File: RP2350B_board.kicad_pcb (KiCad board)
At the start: 2 copper layers, 47.5 x 66 mm, 45 parts, among them IC1 W25Q128JVSIM, IC2 UA78M33CDCYG3, J1 USB_C_Receptacle_USB2.0_16P, J2 SWD, J3 Conn_01x25_Pin, J4 Conn_01x25_Pin, J5 Conn_01x25_Pin, J6 Conn_01x25_Pin, J7 Conn_01x25_Pin, J8 Conn_01x25_Pin, U1 RP2350_80QFN, Y1 ABM8-272-T3

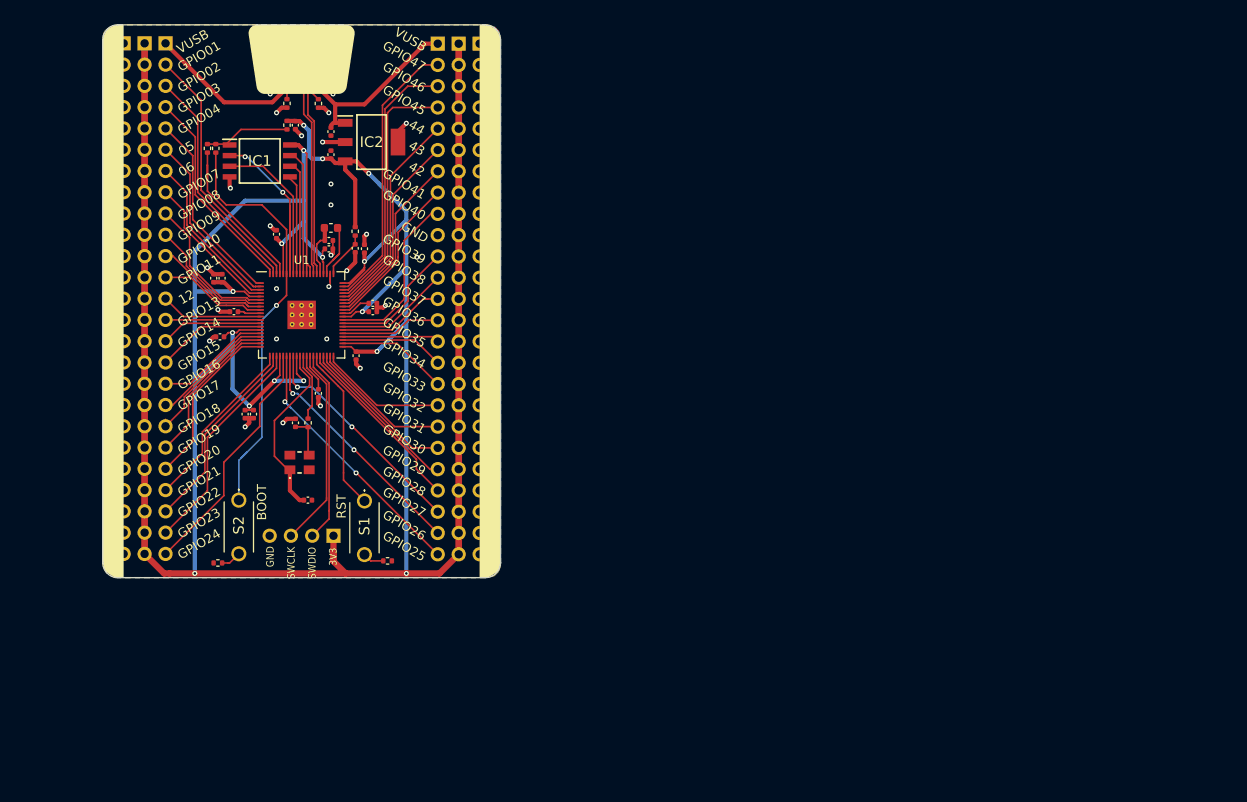
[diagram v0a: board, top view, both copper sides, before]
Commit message: refactor: start new layout
Signed-off-by: Aditya Agarwal <aditya.agarwal030504@gmail.com>
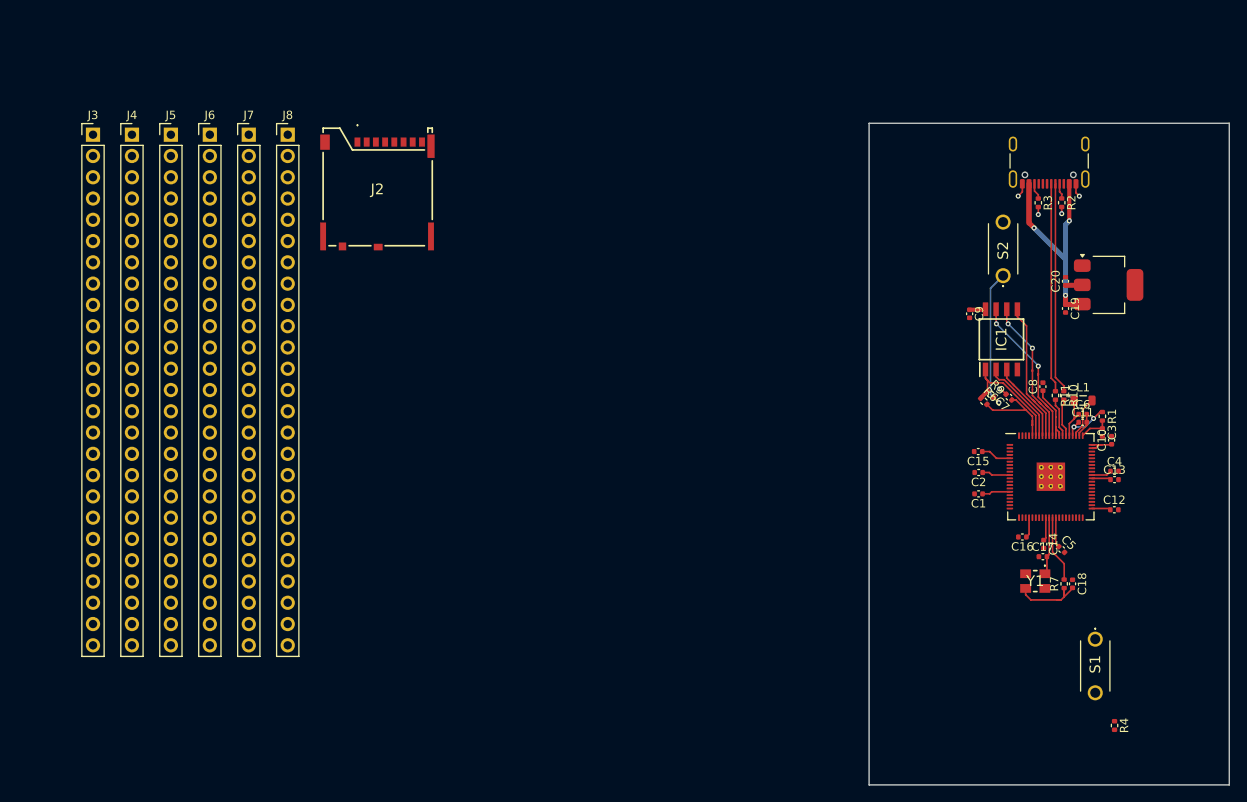
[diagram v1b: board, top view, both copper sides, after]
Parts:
- removed G***: LOGO, Dumblebots-Logo:Dumblebots-Logo
- removed IC2: UA78M33CDCYG3, UA78M33CDCYG3:SOT230P700X180-4N
- removed R5: 0, Resistor_SMD:R_0402_1005Metric
- removed R8: 1K, Resistor_SMD:R_0402_1005Metric
- added R10: 27, Resistor_SMD:R_0402_1005Metric, F.Cu at (237.2, 104.0)
- added R11: 27, Resistor_SMD:R_0402_1005Metric, F.Cu at (236.2, 104.0)
- added U2: NCP1117-3.3_SOT223, Package_TO_SOT_SMD:SOT-223-3_TabPin2, F.Cu at (242.6, 90.8)
- C19, C20: value 100n -> 10u
- J2: value SWD -> MEM2080-00-128-00-A; footprint Connector_PinHeader_2.54mm:PinHeader_1x04_P2.54mm_Vertical -> MEM2080-00-128-00-A:MEM20800012800A
- L1: footprint Inductor_SMD:L_0603_1608Metric -> Inductor_SMD:L_0805_2012Metric
- R4: value 10K -> 1K
- R6: value DNF -> 10K
- moved R4 122.1 mm to (243.3, 143.4), turned to -90 degrees
- moved C13 108.2 mm to (243.3, 114.0), turned to 0 degrees
- moved C12 104.4 mm to (243.3, 117.7), turned to 0 degrees
- moved C14 104.1 mm to (234.8, 121.8), turned to -90 degrees
- moved C6 102.1 mm to (239.5, 106.2), turned to 0 degrees
- moved C16 99.8 mm to (232.3, 120.9), turned to 180 degrees
- moved C11 99.0 mm to (239.5, 107.2), turned to 0 degrees
- moved R6 97.5 mm to (227.7, 104.7), turned to -45 degrees
- moved C3 95.2 mm to (241.8, 108.4), turned to -90 degrees
- moved S2 95.1 mm to (230.0, 89.7), turned to 90 degrees
- moved C18 94.7 mm to (238.3, 126.5), turned to -90 degrees
- moved R9 94.4 mm to (228.5, 103.9), turned to -45 degrees
- moved C15 92.6 mm to (227.0, 110.7), turned to 180 degrees
- moved R7 92.3 mm to (237.3, 126.5)
- moved L1 92.1 mm to (239.6, 104.6)
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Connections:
- net /VREG_LX renamed VREG_LX
- net Net-(U1-XOUT) renamed XOUT
- C1 pad 1: /VREG_AVDD -> IOVDD
- C1 pad 2: GND -> VREG_PGND
- C10 pad 1: +3.3v -> IOVDD
- C10 pad 2: GND -> VREG_PGND
- C11 pad 1: +3.3v -> IOVDD
- C11 pad 2: GND -> VREG_PGND
- C12 pad 1: +3.3v -> IOVDD
- C12 pad 2: GND -> VREG_PGND
- C13 pad 1: +3.3v -> IOVDD
- C13 pad 2: GND -> VREG_PGND
- C14 pad 1: +3.3v -> IOVDD
- C14 pad 2: GND -> VREG_PGND
- C15 pad 1: +3.3v -> IOVDD
- C15 pad 2: GND -> VREG_PGND
- C16 pad 1: +3.3v -> IOVDD
- C16 pad 2: GND -> VREG_PGND
- C17 pad 1: Net-(U1-XIN) -> VREG_PGND
- C17 pad 2: GND -> XIN
- C18 pad 1: Net-(Y1-CRYSTAL_2) -> VREG_PGND
- C18 pad 2: GND -> Net-(C18-Pad2)
- C19 pad 2: GND -> VREG_PGND
- C2 pad 1: +3.3v -> DVDD
- C2 pad 2: GND -> VREG_PGND
- C20 pad 1: GND -> IOVDD
- C20 pad 2: +3.3v -> VREG_PGND
- C3 pad 1: +1V1 -> VREG_AVDD
- C3 pad 2: GND -> VREG_PGND
- C4 pad 1: +1V1 -> DVDD
- C4 pad 2: GND -> VREG_PGND
- C5 pad 1: +1V1 -> DVDD
- C5 pad 2: GND -> VREG_PGND
- C6 pad 1: +1V1 -> DVDD
- C6 pad 2: GND -> VREG_PGND
- C7 pad 1: +3.3v -> IOVDD
- C7 pad 2: GND -> VREG_PGND
- C8 pad 1: +3.3v -> IOVDD
- C8 pad 2: GND -> VREG_PGND
- C9 pad 1: +3.3v -> IOVDD
- C9 pad 2: GND -> VREG_PGND
- IC1 pad 1: Net-(IC1-~{CS}) -> GPIO0
- IC1 pad 4: GND -> VREG_PGND
- IC1 pad 8: +3.3v -> IOVDD
- J1 pad A1: GND -> VREG_PGND
- J1 pad A12: GND -> VREG_PGND
- J1 pad A6: USB_D+ -> Net-(J1-D+-PadA6)
- J1 pad A7: USB_D- -> Net-(J1-D--PadA7)
- J1 pad B1: GND -> VREG_PGND
- J1 pad B12: GND -> VREG_PGND
- J1 pad B6: USB_D+ -> Net-(J1-D+-PadA6)
- J1 pad B7: USB_D- -> Net-(J1-D--PadA7)
- J1 pad S1: GND -> VREG_PGND
- J2 pad 1: +3.3v -> unconnected-(J2-DAT2-Pad1)
- J2 pad 2: SWD -> unconnected-(J2-CD/DAT3-Pad2)
- J2 pad 3: SWCLK -> unconnected-(J2-CMD-Pad3)
- J2 pad 4: GND -> unconnected-(J2-VDD-Pad4)
- J4 pad 10: GND -> VREG_PGND
- J5 pad 1: GND -> VREG_PGND
- J5 pad 10: GND -> VREG_PGND
- J5 pad 11: GND -> VREG_PGND
- J5 pad 12: GND -> VREG_PGND
- J5 pad 13: GND -> VREG_PGND
- J5 pad 14: GND -> VREG_PGND
- J5 pad 15: GND -> VREG_PGND
- J5 pad 16: GND -> VREG_PGND
- J5 pad 17: GND -> VREG_PGND
- J5 pad 18: GND -> VREG_PGND
- J5 pad 19: GND -> VREG_PGND
- J5 pad 2: GND -> VREG_PGND
- J5 pad 20: GND -> VREG_PGND
- J5 pad 21: GND -> VREG_PGND
- J5 pad 22: GND -> VREG_PGND
- J5 pad 23: GND -> VREG_PGND
- J5 pad 24: GND -> VREG_PGND
- J5 pad 25: GND -> VREG_PGND
- J5 pad 3: GND -> VREG_PGND
- J5 pad 4: GND -> VREG_PGND
- J5 pad 5: GND -> VREG_PGND
- J5 pad 6: GND -> VREG_PGND
- J5 pad 7: GND -> VREG_PGND
- J5 pad 8: GND -> VREG_PGND
- J5 pad 9: GND -> VREG_PGND
- J6 pad 1: GND -> VREG_PGND
- J6 pad 10: GND -> VREG_PGND
- J6 pad 11: GND -> VREG_PGND
- J6 pad 12: GND -> VREG_PGND
- J6 pad 13: GND -> VREG_PGND
- J6 pad 14: GND -> VREG_PGND
- J6 pad 15: GND -> VREG_PGND
- J6 pad 16: GND -> VREG_PGND
- J6 pad 17: GND -> VREG_PGND
- J6 pad 18: GND -> VREG_PGND
- J6 pad 19: GND -> VREG_PGND
- J6 pad 2: GND -> VREG_PGND
- J6 pad 20: GND -> VREG_PGND
- J6 pad 21: GND -> VREG_PGND
- J6 pad 22: GND -> VREG_PGND
- J6 pad 23: GND -> VREG_PGND
- J6 pad 24: GND -> VREG_PGND
- J6 pad 25: GND -> VREG_PGND
- J6 pad 3: GND -> VREG_PGND
- J6 pad 4: GND -> VREG_PGND
- J6 pad 5: GND -> VREG_PGND
- J6 pad 6: GND -> VREG_PGND
- J6 pad 7: GND -> VREG_PGND
- J6 pad 8: GND -> VREG_PGND
- J6 pad 9: GND -> VREG_PGND
- J7 pad 1: +3.3v -> IOVDD
- J7 pad 10: +3.3v -> IOVDD
- J7 pad 11: +3.3v -> IOVDD
- J7 pad 12: +3.3v -> IOVDD
- J7 pad 13: +3.3v -> IOVDD
- J7 pad 14: +3.3v -> IOVDD
- J7 pad 15: +3.3v -> IOVDD
- J7 pad 16: +3.3v -> IOVDD
- J7 pad 17: +3.3v -> IOVDD
- J7 pad 18: +3.3v -> IOVDD
- J7 pad 19: +3.3v -> IOVDD
- J7 pad 2: +3.3v -> IOVDD
- J7 pad 20: +3.3v -> IOVDD
- J7 pad 21: +3.3v -> IOVDD
- J7 pad 22: +3.3v -> IOVDD
- J7 pad 23: +3.3v -> IOVDD
- J7 pad 24: +3.3v -> IOVDD
- J7 pad 25: +3.3v -> IOVDD
- J7 pad 3: +3.3v -> IOVDD
- J7 pad 4: +3.3v -> IOVDD
- J7 pad 5: +3.3v -> IOVDD
- J7 pad 6: +3.3v -> IOVDD
- J7 pad 7: +3.3v -> IOVDD
- J7 pad 8: +3.3v -> IOVDD
- J7 pad 9: +3.3v -> IOVDD
- J8 pad 1: +3.3v -> IOVDD
- J8 pad 10: +3.3v -> IOVDD
- J8 pad 11: +3.3v -> IOVDD
- J8 pad 12: +3.3v -> IOVDD
- J8 pad 13: +3.3v -> IOVDD
- J8 pad 14: +3.3v -> IOVDD
- J8 pad 15: +3.3v -> IOVDD
- J8 pad 16: +3.3v -> IOVDD
- J8 pad 17: +3.3v -> IOVDD
- J8 pad 18: +3.3v -> IOVDD
- J8 pad 19: +3.3v -> IOVDD
- J8 pad 2: +3.3v -> IOVDD
- J8 pad 20: +3.3v -> IOVDD
- J8 pad 21: +3.3v -> IOVDD
- J8 pad 22: +3.3v -> IOVDD
- J8 pad 23: +3.3v -> IOVDD
- J8 pad 24: +3.3v -> IOVDD
- J8 pad 25: +3.3v -> IOVDD
- J8 pad 3: +3.3v -> IOVDD
- J8 pad 4: +3.3v -> IOVDD
- J8 pad 5: +3.3v -> IOVDD
- J8 pad 6: +3.3v -> IOVDD
- J8 pad 7: +3.3v -> IOVDD
- J8 pad 8: +3.3v -> IOVDD
- J8 pad 9: +3.3v -> IOVDD
- L1 pad 1: +1V1 -> DVDD
- R1 pad 1: +3.3v -> IOVDD
- R1 pad 2: /VREG_AVDD -> VREG_AVDD
- R2 pad 2: GND -> VREG_PGND
- R3 pad 2: GND -> VREG_PGND
- R4 pad 1: Net-(IC1-~{CS}) -> VREG_PGND
- R4 pad 2: +3.3v -> Net-(S1-NO)
- R6 pad 2: Net-(IC1-~{CS}) -> IOVDD
- R7 pad 1: Net-(Y1-CRYSTAL_2) -> Net-(C18-Pad2)
- R9 pad 1: GND -> GPIO0
- R9 pad 2: Net-(S2-NO) -> Net-(S2-COM)
- S2 pad 1: QSPI_SS -> Net-(S2-COM)
- S2 pad 2: Net-(S2-NO) -> VREG_PGND
- U1 pad 10: +1V1 -> DVDD
- U1 pad 15: +3.3v -> IOVDD
- U1 pad 24: +3.3v -> IOVDD
- U1 pad 29: +3.3v -> IOVDD
- U1 pad 30: Net-(U1-XIN) -> XIN
- U1 pad 32: +1V1 -> DVDD
- U1 pad 41: +3.3v -> IOVDD
- U1 pad 5: +3.3v -> IOVDD
- U1 pad 50: +3.3v -> IOVDD
- U1 pad 51: +1V1 -> DVDD
- U1 pad 59: +3.3v -> IOVDD
- U1 pad 60: +3.3v -> IOVDD
- U1 pad 61: /VREG_AVDD -> VREG_AVDD
- U1 pad 62: GND -> VREG_PGND
- U1 pad 64: +3.3v -> IOVDD
- U1 pad 65: +1V1 -> DVDD
- U1 pad 68: +3.3v -> IOVDD
- U1 pad 69: +3.3v -> IOVDD
- U1 pad 75: QSPI_SS -> GPIO0
- U1 pad 76: +3.3v -> IOVDD
- U1 pad 81: GND -> VREG_PGND
- Y1 pad 1: Net-(U1-XIN) -> XIN
- Y1 pad 2: GND -> VREG_PGND
- Y1 pad 3: Net-(Y1-CRYSTAL_2) -> Net-(C18-Pad2)
- Y1 pad 4: GND -> VREG_PGND
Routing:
- net +3.3v: track 421.7 -> 0.00 mm, vias 16 -> 0
- net QSPI_SS: track 50.9 -> 0.00 mm, vias 1 -> 0
- net IOVDD: track 0.00 -> 48.8 mm, vias 0 -> 2
- net GND: track 37.4 -> 0.00 mm, vias 27 -> 0
- net GPIO47: track 33.0 -> 0.00 mm
- net GPIO25: track 32.1 -> 0.00 mm, vias 2 -> 0
- net GPIO46: track 31.9 -> 0.00 mm
- net GPIO45: track 30.8 -> 0.00 mm
- net GPIO1: track 30.5 -> 0.00 mm
- net GPIO26: track 30.3 -> 0.00 mm, vias 2 -> 0
- net GPIO24: track 29.5 -> 0.00 mm
- net GPIO2: track 27.8 -> 0.00 mm
- net GPIO27: track 26.8 -> 0.00 mm, vias 2 -> 0
- net GPIO23: track 26.6 -> 0.00 mm
- net GPIO44: track 25.6 -> 0.00 mm
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- removed copper zone on B.Cu, net GND
- removed copper zone on F.Cu, net GND
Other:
- board size 47.5 x 66 mm -> 43 x 79 mm
- board text removed: "05"
- board text removed: "06"
- board text removed: "12"
- board text removed: "3V3"
- board text removed: "42"
- board text removed: "43"
- board text removed: "44"
- board text removed: "BOOT"
- board text removed: "Designed and manufactured in Bharat"
- board text removed: "GND"
- board text removed: "GPIO01"
- board text removed: "GPIO02"
- board text removed: "GPIO03"
- board text removed: "GPIO04"
- board text removed: "GPIO07"
- board text removed: "GPIO08"
- board text removed: "GPIO09"
- board text removed: "GPIO10"
- board text removed: "GPIO11"
- board text removed: "GPIO13"
- board text removed: "GPIO14"
- board text removed: "GPIO15"
- board text removed: "GPIO16"
- board text removed: "GPIO17"
- board text removed: "GPIO18"
- board text removed: "GPIO19"
- board text removed: "GPIO20"
- board text removed: "GPIO21"
- board text removed: "GPIO22"
- board text removed: "GPIO23"
- board text removed: "GPIO24"
- board text removed: "GPIO25"
- board text removed: "GPIO26"
- board text removed: "GPIO27"
- board text removed: "GPIO28"
- board text removed: "GPIO29"
- board text removed: "GPIO30"
- board text removed: "GPIO31"
- board text removed: "GPIO32"
- board text removed: "GPIO33"
- board text removed: "GPIO34"
- board text removed: "GPIO35"
- board text removed: "GPIO36"
- board text removed: "GPIO37"
- board text removed: "GPIO38"
- board text removed: "GPIO39"
- board text removed: "GPIO40"
- board text removed: "GPIO41"
- board text removed: "GPIO45"
- board text removed: "GPIO46"
- board text removed: "GPIO47"
- board text removed: "RP2350B Dev Board"
- board text removed: "RST"
- board text removed: "SWCLK"
- board text removed: "SWDIO"
- board text removed: "VUSB"
- board text removed: "dumblebots.com"

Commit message: feat: complete all features except SD Card reader
Signed-off-by: Aditya Agarwal <aditya.agarwal030504@gmail.com>
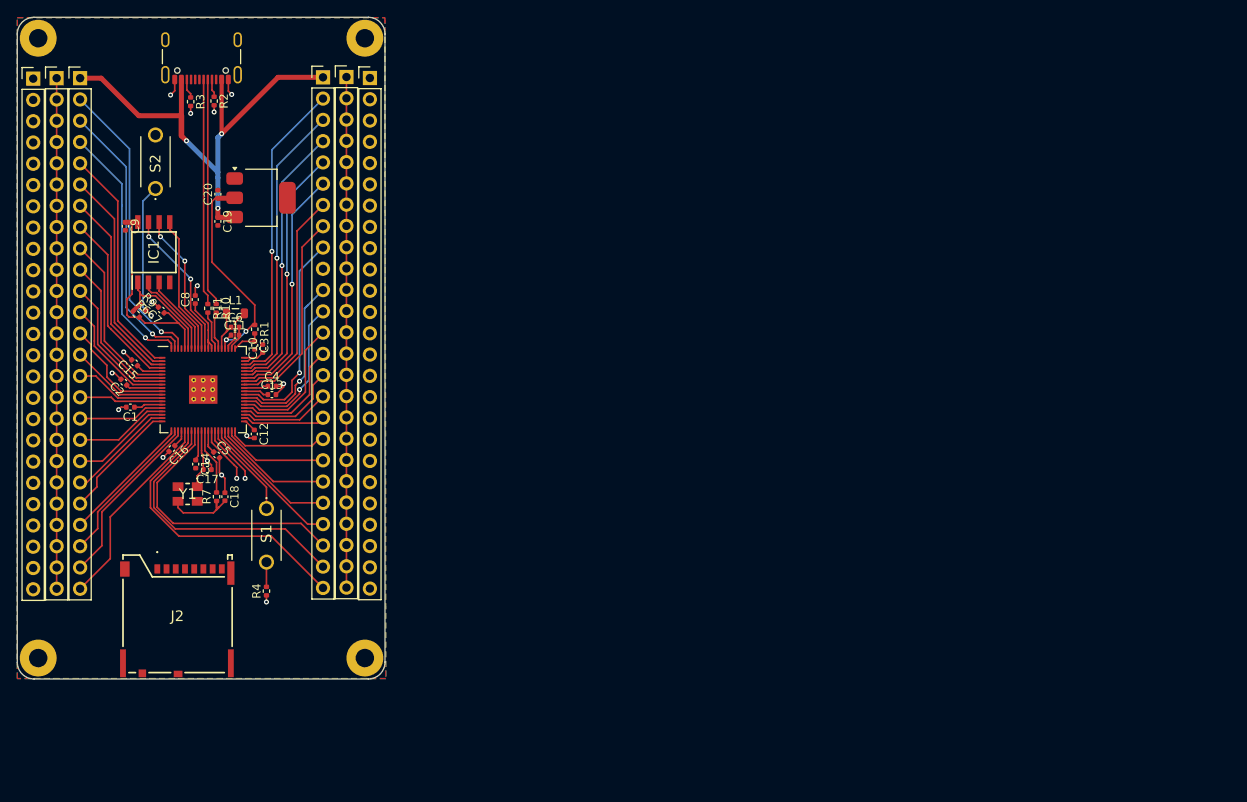
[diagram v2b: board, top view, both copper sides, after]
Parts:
- added REF**: MountingHole_2.2mm_M2_Pad, MountingHole:MountingHole_2.2mm_M2_Pad, F.Cu at (153.8, 135.3)
- added REF**: MountingHole_2.2mm_M2_Pad, MountingHole:MountingHole_2.2mm_M2_Pad, F.Cu at (114.8, 135.3)
- added REF**: MountingHole_2.2mm_M2_Pad, MountingHole:MountingHole_2.2mm_M2_Pad, F.Cu at (153.8, 61.4)
- added REF**: MountingHole_2.2mm_M2_Pad, MountingHole:MountingHole_2.2mm_M2_Pad, F.Cu at (114.8, 61.4)
- moved C12 103.1 mm to (140.6, 108.6), turned to -90 degrees
- moved C2 102.6 mm to (125.0, 102.4), turned to 135 degrees
- moved R4 102.5 mm to (142.1, 127.4), turned to 90 degrees
- moved C16 102.1 mm to (130.8, 110.3), turned to -135 degrees
- moved J1 102.0 mm to (134.3, 62.6)
- moved C10 101.9 mm to (141.6, 98.4)
- moved R2 101.9 mm to (135.8, 68.8)
- moved R3 101.9 mm to (133.0, 68.9)
- moved C1 101.8 mm to (125.8, 105.4)
- moved IC1 101.7 mm to (128.6, 86.9)
- moved L1 101.7 mm to (138.3, 94.2)
- moved Y1 101.7 mm to (132.6, 115.8)
- moved R9 101.7 mm to (127.3, 93.5)
- moved C11 101.7 mm to (138.3, 96.8)
- moved C18 101.7 mm to (137.1, 116.1)
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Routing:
- net IOVDD: track 48.8 -> 200.8 mm
- net GPIO47: track 0.00 -> 36.9 mm, vias 0 -> 1
- net GPIO25: track 0.00 -> 35.6 mm
- net GPIO1: track 0.00 -> 35.3 mm, vias 0 -> 1
- net GPIO46: track 0.00 -> 34.8 mm, vias 0 -> 1
- net GPIO26: track 0.00 -> 34.2 mm
- net GPIO2: track 0.00 -> 33.0 mm, vias 0 -> 1
- net VBUS: track 28.1 -> 61.0 mm
- net GPIO45: track 0.00 -> 32.8 mm, vias 0 -> 1
- net GPIO27: track 0.00 -> 32.7 mm
- net GPIO44: track 0.00 -> 31.1 mm, vias 0 -> 1
- net GPIO3: track 0.00 -> 30.6 mm, vias 0 -> 1
- net GPIO43: track 0.00 -> 28.7 mm, vias 0 -> 1
- net GPIO4: track 0.00 -> 27.8 mm
- net GPIO42: track 0.00 -> 26.7 mm
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- added copper zone on B.Cu, net VREG_PGND
- added copper zone on F.Cu, net VREG_PGND
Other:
- board size 43 x 79 mm -> 43.9 x 79 mm
